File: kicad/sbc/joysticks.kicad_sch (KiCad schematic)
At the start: 8 parts, among them U28 7400, U29 74LS244, U7 74125

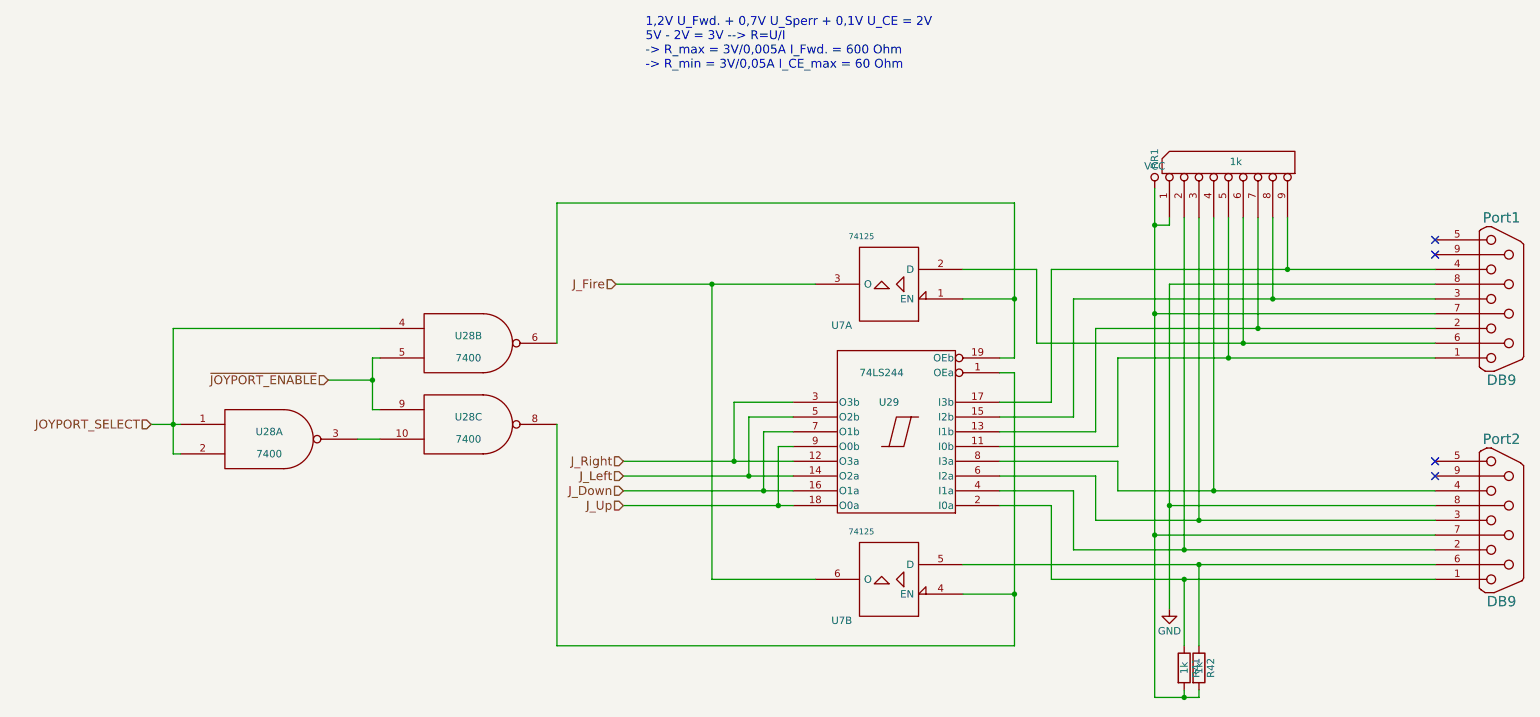
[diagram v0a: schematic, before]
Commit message: routing
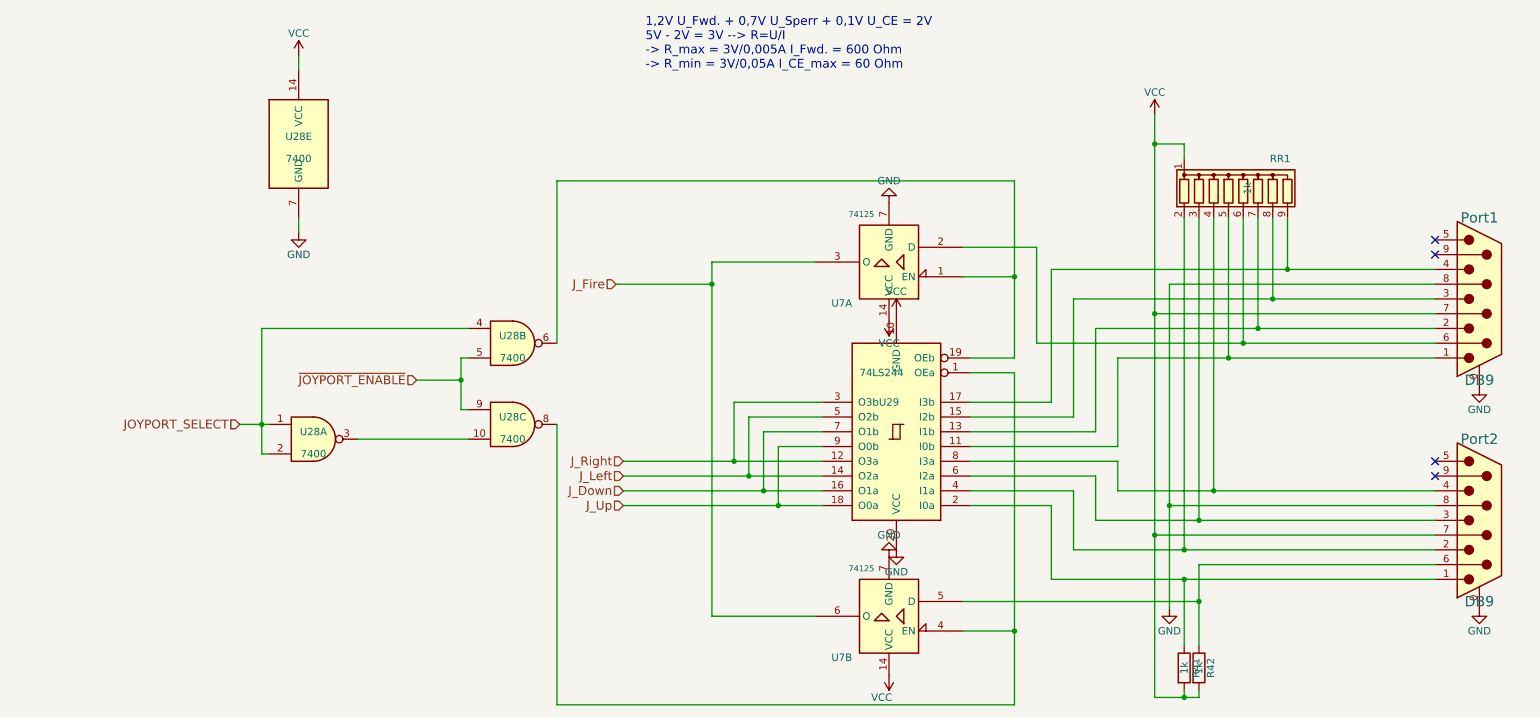
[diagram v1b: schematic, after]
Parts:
- added unit 5 of U28
- Port1, Port2: symbol io-rescue:DB9 -> Connector:DE9_Plug_MountingHoles
- R41, R42: symbol io-rescue:R -> Device:R
- RR1: footprint Resistor_THT:R_Array_SIP8 -> Resistor_THT:R_Array_SIP9; symbol io-rescue:RR8 -> Device:R_Network08
- U28: symbol io-rescue:7400 -> 74xx:7400
- U29: symbol io-rescue:74LS244 -> 74xx:74LS244
- U7: symbol io-rescue:74125 -> 74xx_IEEE:74125
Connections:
- net GND: now also Port1.0 (PAD), Port2.0 (PAD), U29.20 (VCC), U28.7 (GND); no longer U28.7 (GND), U28.7 (GND), U28.7 (GND), U29.10 (GND)
- net VCC: now also U29.10 (GND), U28.14 (VCC); no longer U28.14 (VCC), U28.14 (VCC), U28.14 (VCC), U29.20 (VCC)
